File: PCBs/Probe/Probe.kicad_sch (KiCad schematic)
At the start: 23 parts, among them J1 RS485, J2 Au2, J3 Ti2, J4 Au1, J5 Au3, J6 Ti1, J7 Ti3, Q1 PMOS, U1 SP3485EN

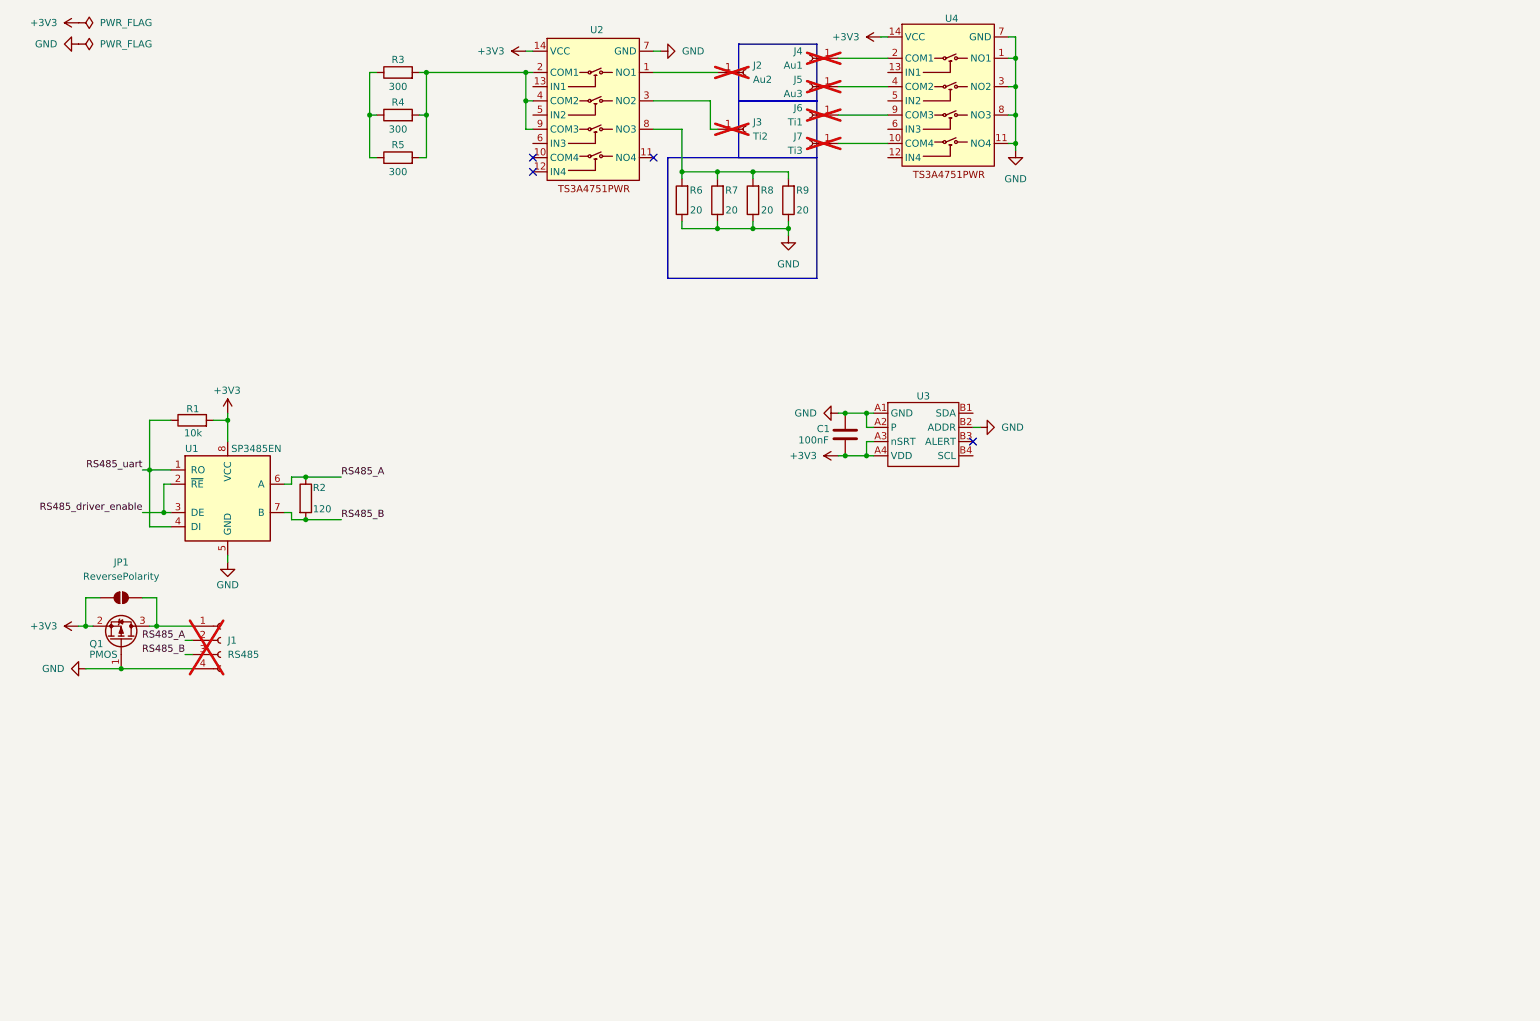
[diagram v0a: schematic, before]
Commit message: pcb work
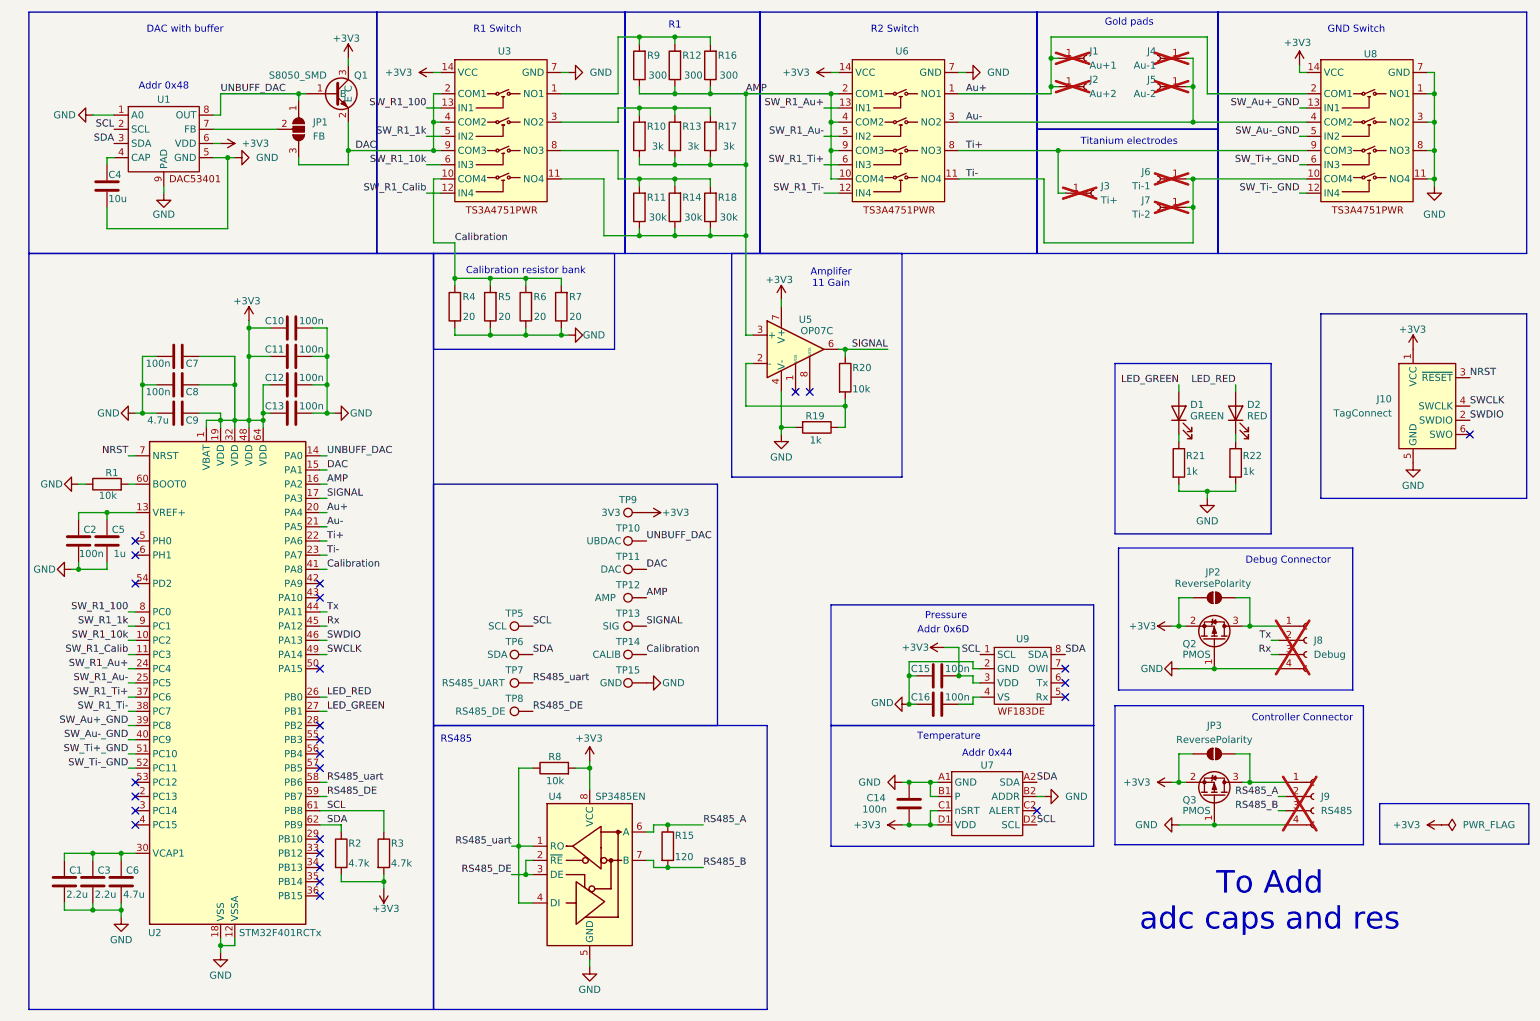
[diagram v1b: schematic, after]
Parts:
- removed R4, R5: 300, symbol Device:R
- added C1, C3: 2.2u, Capacitor_SMD:C_0603_1608Metric, symbol Device:C
- added C10, C11, C12, C13, C15, C16, C2, C7, C8: 100n, Capacitor_SMD:C_0603_1608Metric, symbol Device:C
- added C4: 10u, Capacitor_SMD:C_0603_1608Metric, symbol Device:C
- added C5: 1u, Capacitor_SMD:C_0603_1608Metric, symbol Device:C
- added C6, C9: 4.7u, Capacitor_SMD:C_0603_1608Metric, symbol Device:C
- added D1: GREEN, LED_SMD:LED_0805_2012Metric, symbol Device:LED
- added D2: RED, LED_SMD:LED_0603_1608Metric, symbol Device:LED
- added J10: TagConnect, Connector:Tag-Connect_TC2030-IDC-NL_2x03_P1.27mm_Vertical, symbol Connector:Conn_ARM_SWD_TagConnect_TC2030-NL
- added J2: Au+2, 4022S:Au_Electrode, symbol Connector:Conn_01x01_Socket
- added J8: Debug, Connector_PinSocket_2.54mm:PinSocket_1x04_P2.54mm_Vertical, symbol Connector:Conn_01x04_Socket
- added JP1: FB, Jumper:SolderJumper-3_P2.0mm_Open_TrianglePad1.0x1.5mm, symbol Jumper:SolderJumper_3_Open
- added JP2: ReversePolarity, Jumper:SolderJumper-2_P1.3mm_Open_TrianglePad1.0x1.5mm, symbol Jumper:SolderJumper_2_Open
- added Q1: S8050_SMD, Package_TO_SOT_SMD:SOT-23-3, symbol MyDevices:S8050_SMD
- added Q2: PMOS, Package_TO_SOT_SMD:SOT-23, symbol Transistor_FET:AO3401A
- added R1: 10k, Resistor_SMD:R_0603_1608Metric, symbol Device:R
- added R10, R13, R17: 3k, Resistor_SMD:R_0603_1608Metric, symbol Device:R
- added R11, R14, R18: 30k, Resistor_SMD:R_0603_1608Metric, symbol Device:R
- added R12, R16: 300, Resistor_SMD:R_0603_1608Metric, symbol Device:R
- added R19: 1k, Resistor_SMD:R_1206_3216Metric, symbol Device:R
- added R2, R3: 4.7k, Resistor_SMD:R_0603_1608Metric, symbol Device:R
- added R20: 10k, Resistor_SMD:R_1206_3216Metric, symbol Device:R
- added R21, R22: 1k, Resistor_SMD:R_0603_1608Metric, symbol Device:R
- added TP10: UBDAC, TestPoint:TestPoint_THTPad_2.0x2.0mm_Drill1.0mm, symbol Connector:TestPoint
- added TP11: DAC, TestPoint:TestPoint_THTPad_2.0x2.0mm_Drill1.0mm, symbol Connector:TestPoint
- added TP12: AMP, TestPoint:TestPoint_THTPad_2.0x2.0mm_Drill1.0mm, symbol Connector:TestPoint
- added TP13: SIG, TestPoint:TestPoint_THTPad_2.0x2.0mm_Drill1.0mm, symbol Connector:TestPoint
- added TP14: CALIB, TestPoint:TestPoint_THTPad_2.0x2.0mm_Drill1.0mm, symbol Connector:TestPoint
- added TP15: GND, TestPoint:TestPoint_THTPad_2.0x2.0mm_Drill1.0mm, symbol Connector:TestPoint
- added TP5: SCL, TestPoint:TestPoint_THTPad_2.0x2.0mm_Drill1.0mm, symbol Connector:TestPoint
- added TP6: SDA, TestPoint:TestPoint_THTPad_2.0x2.0mm_Drill1.0mm, symbol Connector:TestPoint
- added TP7: RS485_UART, TestPoint:TestPoint_THTPad_2.0x2.0mm_Drill1.0mm, symbol Connector:TestPoint
- added TP8: RS485_DE, TestPoint:TestPoint_THTPad_2.0x2.0mm_Drill1.0mm, symbol Connector:TestPoint
- added TP9: 3V3, TestPoint:TestPoint_THTPad_2.0x2.0mm_Drill1.0mm, symbol Connector:TestPoint
- added U1: ~, Package_SON:WSON-8-1EP_2x2mm_P0.5mm_EP0.9x1.6mm, symbol 4022S:DAC53401
- added U2: STM32F401RCTx, Package_QFP:LQFP-64_10x10mm_P0.5mm, symbol MCU_ST_STM32F4:STM32F401RCTx
- added U3: ~, Package_SO:TSSOP-14_4.4x5mm_P0.65mm, symbol 4022S:TS3A4751PWR
- added U5: OP07C, Package_SO:SOIC-8_3.9x4.9mm_P1.27mm, symbol Amplifier_Operational:OP07
- added U9: ~, 4022S:WF183DE, symbol 4022S:WF183DE
- C14: renamed from C1; value 100nF -> 100n; footprint (none) -> Capacitor_SMD:C_0603_1608Metric; Cost (none) -> 0,0021; Extended (none) -> False; JLC Part no. (none) -> C14663
- J1: renamed from J2; value Au2 -> Au+1; footprint (none) -> 4022S:Au_Electrode
- J3: value Ti2 -> Ti+; footprint (none) -> Connector_PinHeader_2.54mm:PinHeader_1x01_P2.54mm_Vertical
- J4: value Au1 -> Au-1; footprint (none) -> 4022S:Au_Electrode
- J5: value Au3 -> Au-2; footprint (none) -> 4022S:Au_Electrode
- J6: value Ti1 -> Ti-1; footprint (none) -> Connector_PinHeader_2.54mm:PinHeader_1x01_P2.54mm_Vertical
- J7: value Ti3 -> Ti-2; footprint (none) -> Connector_PinHeader_2.54mm:PinHeader_1x01_P2.54mm_Vertical
- J9: renamed from J1; footprint (none) -> Connector_PinSocket_2.54mm:PinSocket_1x04_P2.54mm_Vertical
- JP3: renamed from JP1; footprint (none) -> Jumper:SolderJumper-2_P1.3mm_Open_TrianglePad1.0x1.5mm
- Q3: renamed from Q1; footprint AnchorRSSA:SOT-23_L2.9-W1.3-P1.90-LS2.4-BR -> Package_TO_SOT_SMD:SOT-23
- R15: renamed from R2; footprint AnchorRSSA:R1206 -> Resistor_SMD:R_0603_1608Metric; Cost 0,0028 -> 0,0010; JLC Part no. C17909 -> C22787
- R4: renamed from R6; footprint (none) -> Resistor_SMD:R_0603_1608Metric; Cost (none) -> 0,0009; Extended (none) -> False; JLC Part no. C17955 -> C22950
- R5: renamed from R7; footprint (none) -> Resistor_SMD:R_0603_1608Metric; Cost (none) -> 0,0009; Extended (none) -> False; JLC Part no. C17955 -> C22950
- R6: renamed from R8; footprint (none) -> Resistor_SMD:R_0603_1608Metric; Cost (none) -> 0,0009; Extended (none) -> False; JLC Part no. C17955 -> C22950
- R7: renamed from R9; footprint (none) -> Resistor_SMD:R_0603_1608Metric; Cost (none) -> 0,0009; Extended (none) -> False; JLC Part no. C17955 -> C22950
- R8: renamed from R1; footprint (none) -> Resistor_SMD:R_0603_1608Metric; Cost (none) -> 0,0008; Extended (none) -> False; JLC Part no. (none) -> C25804
- R9: renamed from R3; footprint (none) -> Resistor_SMD:R_0603_1608Metric; Cost (none) -> 0,0010; Extended (none) -> False; JLC Part no. C17887 -> C23025
- U4: renamed from U1; footprint AnchorRSSA:SOIC-8_L5.0-W4.0-P1.27-LS6.0-BL -> Package_SO:SOIC-8_3.9x4.9mm_P1.27mm
- U6: renamed from U2; footprint (none) -> Package_SO:TSSOP-14_4.4x5mm_P0.65mm; Cost (none) -> 1,4775; Extended (none) -> True; JLC Part no. (none) -> C128399
- U7: renamed from U3; footprint (none) -> Package_CSP:WLCSP-8_1.551x2.284mm_P0.5mm; Cost (none) -> 0,5325; Extended (none) -> True; JLC Part no. (none) -> C2758003
- U8: renamed from U4; footprint (none) -> Package_SO:TSSOP-14_4.4x5mm_P0.65mm; Cost (none) -> 1,4775; Extended (none) -> True; JLC Part no. (none) -> C128399
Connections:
- net +3V3: now also U7.C1 (nSRT), U7.D1 (VDD), C10.1, C11.1, C12.1, C13.1, C15.2, C7.1, C8.1, C9.1, J10.1 (VCC), JP2.1 (A), Q1.3 (C), Q2.2 (S), R2.2, R3.2, TP9.1, U1.6 (VDD), U2.1 (VBAT), U2.19 (VDD), U2.32 (VDD), U2.48 (VDD), U2.64 (VDD), U3.14 (VCC), U5.7 (V+), U9.3 (VDD); no longer U7.A3 (nSRT), U7.A4 (VDD)
- net GND: now also U7.B1 (P), C1.1, C10.2, C11.2, C12.2, C13.2, C15.1, C16.1, C2.1, C3.1, C4.2, C5.1, C6.1, C7.2, C8.2, C9.2, J10.5 (GND), J8.4 (Pin_4), Q2.1 (G), R1.1, R19.2, R21.2, R22.2, TP15.1, U1.1 (A0), U1.5 (GND), U1.9 (PAD), U2.12 (VSSA), U2.18 (VSS), U2.31 (VSS), U2.47 (VSS), U2.63 (VSS), U3.7 (GND), U5.4 (V-), U9.2 (GND); no longer U7.A2 (P)
- net RS485_uart: now also TP7.1, U2.58 (PB6)
- net Au+: now reaches J1.1 (Pin_1), U6.1 (NO1)
- net Au+: now also U8.2 (COM1), J2.1 (Pin_1), U2.20 (PA4)
- net AMP: now reaches U6.10 (COM4)
- net AMP: now also R9.1, U6.2 (COM1), U6.4 (COM2), U6.9 (COM3), R10.1, R11.1, R12.1, R13.1, R14.1, R16.1, R17.1, R18.1, TP12.1, U2.16 (PA2), U3.11 (NO4), U5.3 (+)
- net Ti-: now reaches U6.11 (NO4)
- net Ti-: now also J6.1 (Pin_1), J7.1 (Pin_1), U8.10 (COM4), U2.23 (PA7)
- net SW_R1_Ti-: now reaches U6.12 (IN4)
- net SW_R1_Ti-: now also U2.38 (PC7)
- net SW_R1_Au+: now reaches U6.13 (IN1)
- net SW_R1_Au+: now also U2.24 (PC4)
- net Au-: now reaches U6.3 (NO2)
- net Au-: now also J4.1 (Pin_1), J5.1 (Pin_1), U8.4 (COM2), U2.21 (PA5); no longer J3.1 (Pin_1)
- net SW_R1_Au-: now reaches U6.5 (IN2)
- net SW_R1_Au-: now also U2.25 (PC5)
- net SW_R1_Ti+: now reaches U6.6 (IN3)
- net SW_R1_Ti+: now also U2.37 (PC6)
- net Calibration: now reaches R4.2, R5.2, R6.2, R7.2
- net Calibration: now also TP14.1, U2.41 (PA8), U3.10 (COM4); no longer U6.8 (NO3)
- net SW_Ti-_GND: now reaches U8.12 (IN4)
- net SW_Ti-_GND: now also U2.52 (PC11)
- net SW_Au+_GND: now reaches U8.13 (IN1)
- net SW_Au+_GND: now also U2.39 (PC8)
- net SW_Au-_GND: now reaches U8.5 (IN2)
- net SW_Au-_GND: now also U2.40 (PC9)
- net SW_Ti+_GND: now reaches U8.6 (IN3)
- net SW_Ti+_GND: now also U2.51 (PC10)
- net Ti+: now reaches U8.9 (COM3)
- net Ti+: now also J3.1 (Pin_1), U6.8 (NO3), U2.22 (PA6); no longer J6.1 (Pin_1)
- net RS485_driver_enable renamed RS485_DE
- net RS485_DE: now also TP8.1, U2.59 (PB7)
- new net: R1.2, U2.60 (BOOT0)
- new net: R12.2, R16.2, R9.2, U3.1 (NO1)
- new net: J8.1 (Pin_1), JP2.2 (B), Q2.3 (D)
- new net: R19.1, R20.2, U5.2 (-)
- new net: R10.2, R13.2, R17.2, U3.3 (NO2)
- new net: C4.1, U1.4 (CAP)
- new net: JP1.2 (C), U1.7 (FB)
- new net: D1.1 (K), R21.1
- new net: C1.2, C3.2, C6.2, U2.30 (VCAP1)
- new net: R11.2, R14.2, R18.2, U3.8 (NO3)
- new net: C16.2, U9.4 (VS)
- new net: D2.1 (K), R22.1
- new net: C2.2, C5.2, U2.13 (VREF+)
- new net DAC: JP1.3 (B), Q1.2 (E), TP11.1, U2.15 (PA1), U3.2 (COM1), U3.4 (COM2), U3.9 (COM3)
- new net LED_GREEN: D1.2 (A), U2.27 (PB1)
- new net LED_RED: D2.2 (A), U2.26 (PB0)
- new net NRST: J10.3 (~{RESET}), U2.7 (NRST)
- new net Rx: J8.3 (Pin_3), U2.45 (PA12)
- new net SCL: R3.1, TP5.1, U1.2 (SCL), U2.61 (PB8), U7.D2 (SCL), U9.1 (SCL)
- new net SDA: R2.1, TP6.1, U1.3 (SDA), U2.62 (PB9), U7.A2 (SDA), U9.8 (SDA)
- new net SIGNAL: R20.1, TP13.1, U2.17 (PA3), U5.6
- new net SWCLK: J10.4 (SWCLK), U2.49 (PA14)
- new net SWDIO: J10.2 (SWDIO), U2.46 (PA13)
- new net SW_R1_100: U2.8 (PC0), U3.13 (IN1)
- new net SW_R1_10k: U2.10 (PC2), U3.6 (IN3)
- new net SW_R1_1k: U2.9 (PC1), U3.5 (IN2)
- new net SW_R1_Calib: U2.11 (PC3), U3.12 (IN4)
- new net Tx: J8.2 (Pin_2), U2.44 (PA11)
- new net UNBUFF_DAC: JP1.1 (A), Q1.1 (B), TP10.1, U1.8 (OUT), U2.14 (PA0)
- no-connect marks 4 -> 26
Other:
- note added: "Addr 0x44"
- note added: "Addr 0x48"
- note added: "Addr 0x6D"
- note added: "Amplifer 11 Gain"
- note added: "Calibration resistor bank"
- note added: "Controller Connector"
- note added: "DAC with buffer"
- note added: "Debug Connector"
- note added: "GND Switch"
- note added: "Gold pads"
- note added: "Pressure"
- note added: "R1"
- note added: "R1 Switch"
- note added: "R2 Switch"
- note added: "RS485"
- note added: "Temperature"
- note added: "Titanium electrodes"
- note added: "To Add adc caps and res"
- company: (none) -> University of Cape Town
- title: (none) -> Salinity Prode
- moved on the sheet: C14, J1, J3, J4, J5, J6, J7, J9, JP3, Q3, R15, R4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
